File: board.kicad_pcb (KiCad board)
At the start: 4 copper layers, 50 x 50 mm, 47 parts, among them J1 TEMPS, J2 OLED, J3 HV1, J4 HV2, J5 PWR_IN, J6 PROG, K1 RELAY1, K3 RELAY2, Q3 AO3400A, Q4 AO3400A, U1 ESP32-WROOM-32, U2 AMS1117, U3 USB3_1C16PFSMT, U4 CH340E, U5 SW_RST, U6 SW_BOOT

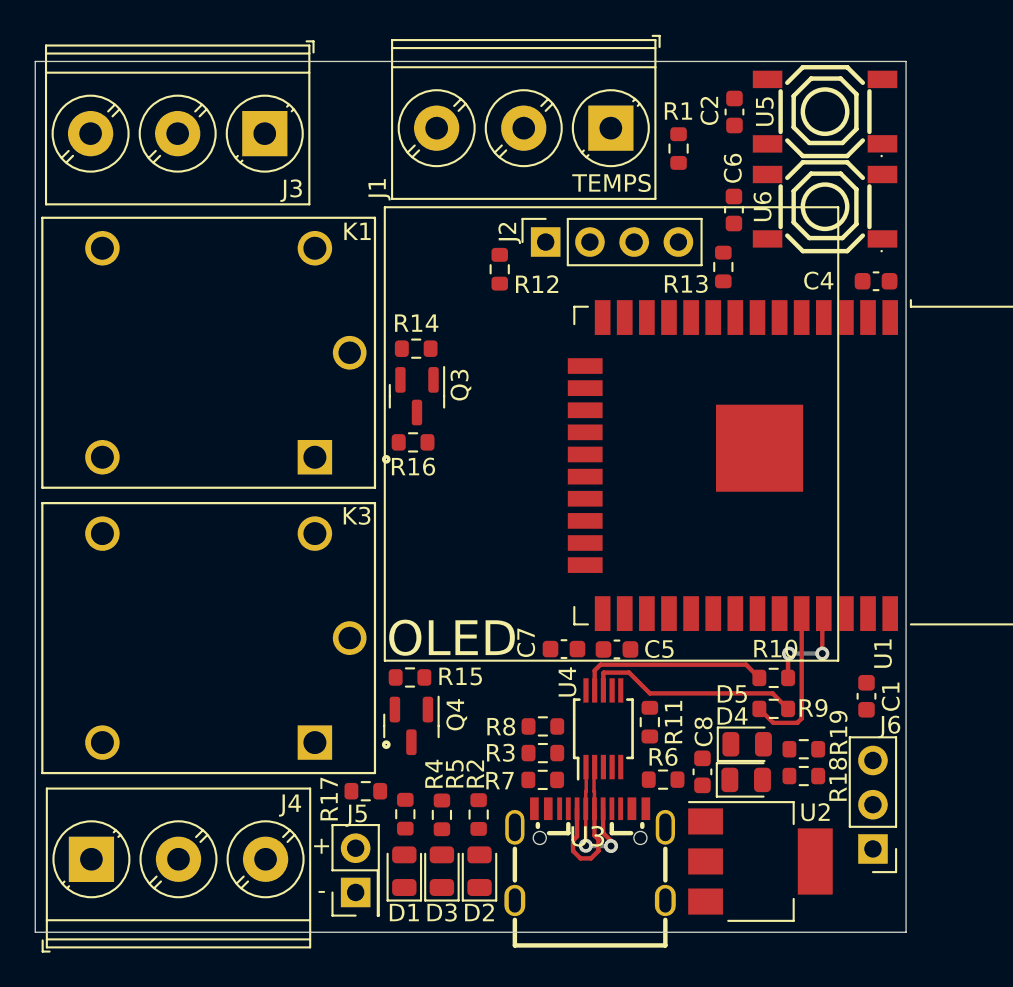
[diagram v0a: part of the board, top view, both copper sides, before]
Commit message: feat: initial routing
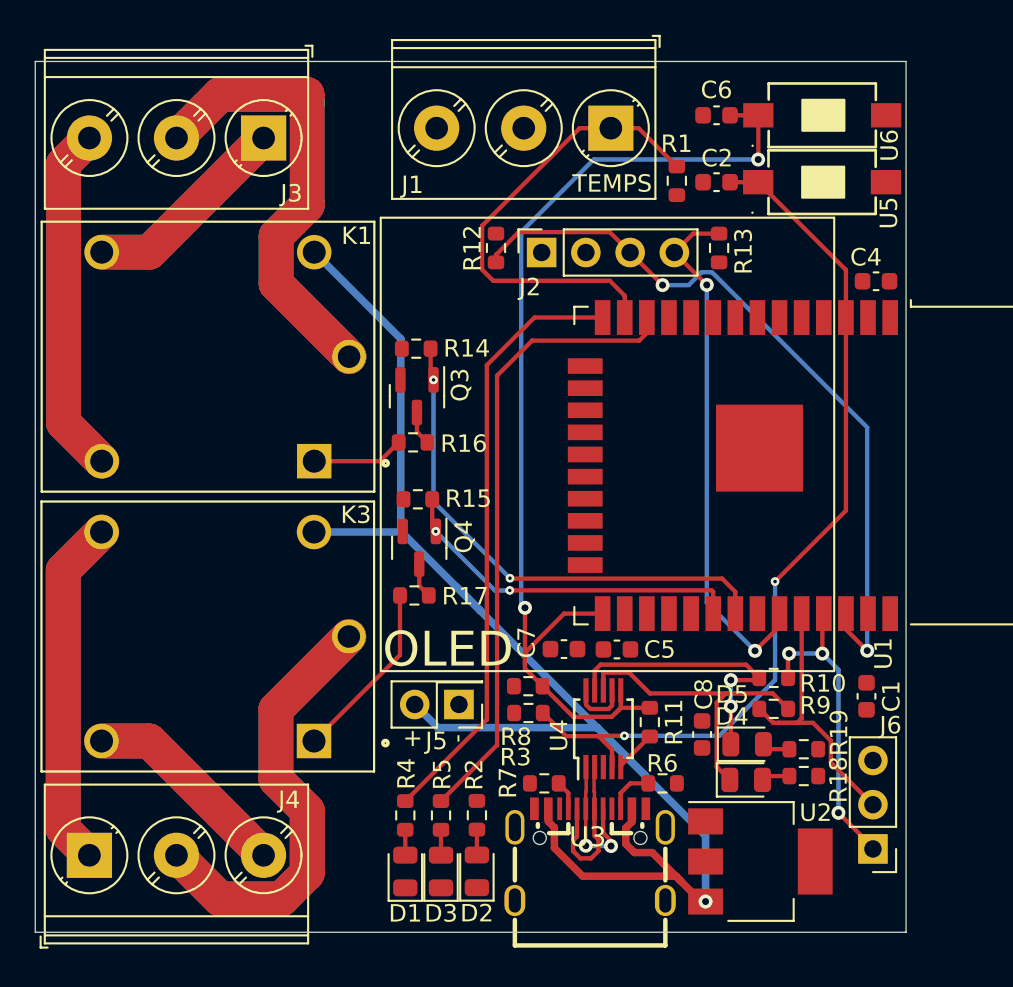
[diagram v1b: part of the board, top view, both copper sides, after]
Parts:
- J3: value HV1 -> HV2
- J4: value HV2 -> HV1
- K1: value RELAY1 -> RELAY2
- K3: value RELAY2 -> RELAY1
- U2: value AMS1117 -> AMS1117-3.3
- U5, U6: footprint board:SW-SMD_4P-L5.1-W5.1-P3.70-LS6.5-TL-2 -> board:SW-SMD_L6.0-W3.5-LS8.0
- moved J5 12.3 mm to (78.8, 140.2), turned to 180 degrees
- moved R17 11.6 mm to (76.3, 133.9)
- moved Q4 10.2 mm to (76.5, 131.2)
- moved R15 10.2 mm to (76.5, 128.4)
- moved C6 5.53 mm to (93.6, 106.4), turned to 0 degrees
- moved U6 5.25 mm to (99.7, 106.4), turned to 0 degrees
- moved C2 4.16 mm to (93.6, 110.2), turned to 0 degrees
- moved U5 4.05 mm to (99.7, 110.2), turned to 0 degrees
- moved R8 2.46 mm to (82.8, 139.2)
- moved R3 2.45 mm to (82.8, 140.7)
- moved C8 2.15 mm to (92.8, 141.9)
- moved R1 1.85 mm to (91.3, 110.1)
- moved R12 1.24 mm to (81.0, 114.0)
- moved R13 1.12 mm to (93.8, 114.0)
- moved J2 0.64 mm to (83.6, 114.3)
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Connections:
- Q3 pad 1: CH1 -> CH2
- Q4 pad 1: CH2 -> CH1
- R14 pad 2: CH1 -> CH2
- R15 pad 2: CH2 -> CH1
- U5 pad 2: EN_ESP -> GND
- U6 pad 2: GPIO0 -> GND
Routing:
- net Net-(J3-Pad2): track 0.00 -> 103.2 mm
- net Net-(J4-Pad2): track 0.00 -> 100.9 mm
- net VBUS: track 0.00 -> 87.0 mm, vias 0 -> 1
- net Net-(J4-Pad1): track 0.00 -> 80.4 mm
- net Net-(J3-Pad3): track 0.00 -> 80.3 mm
- net GPIO0: track 0.00 -> 60.6 mm, vias 0 -> 2
- net EN_ESP: track 0.00 -> 51.3 mm, vias 0 -> 2
- net Net-(J4-Pad3): track 0.00 -> 48.1 mm
- net Net-(J3-Pad1): track 0.00 -> 48.0 mm
- net SCL: track 0.00 -> 43.0 mm, vias 0 -> 2
- net SLED2: track 0.00 -> 36.3 mm
- net SLED1: track 0.00 -> 34.7 mm
- net SDA: track 0.00 -> 30.5 mm, vias 0 -> 2
- net CH2: track 0.00 -> 29.6 mm, vias 0 -> 2
- net GPIO14: track 0.00 -> 27.0 mm
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
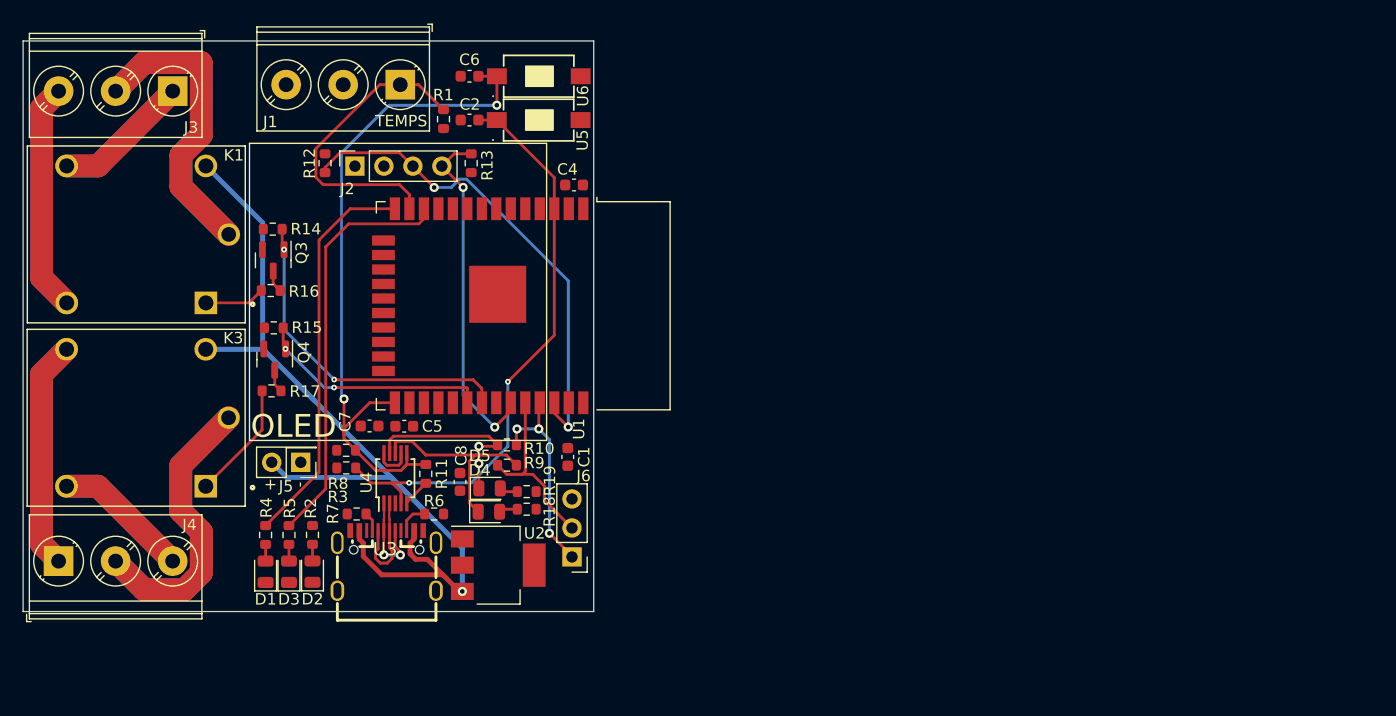
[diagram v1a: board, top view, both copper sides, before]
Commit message: feat: routed with planes and no warnings or errors
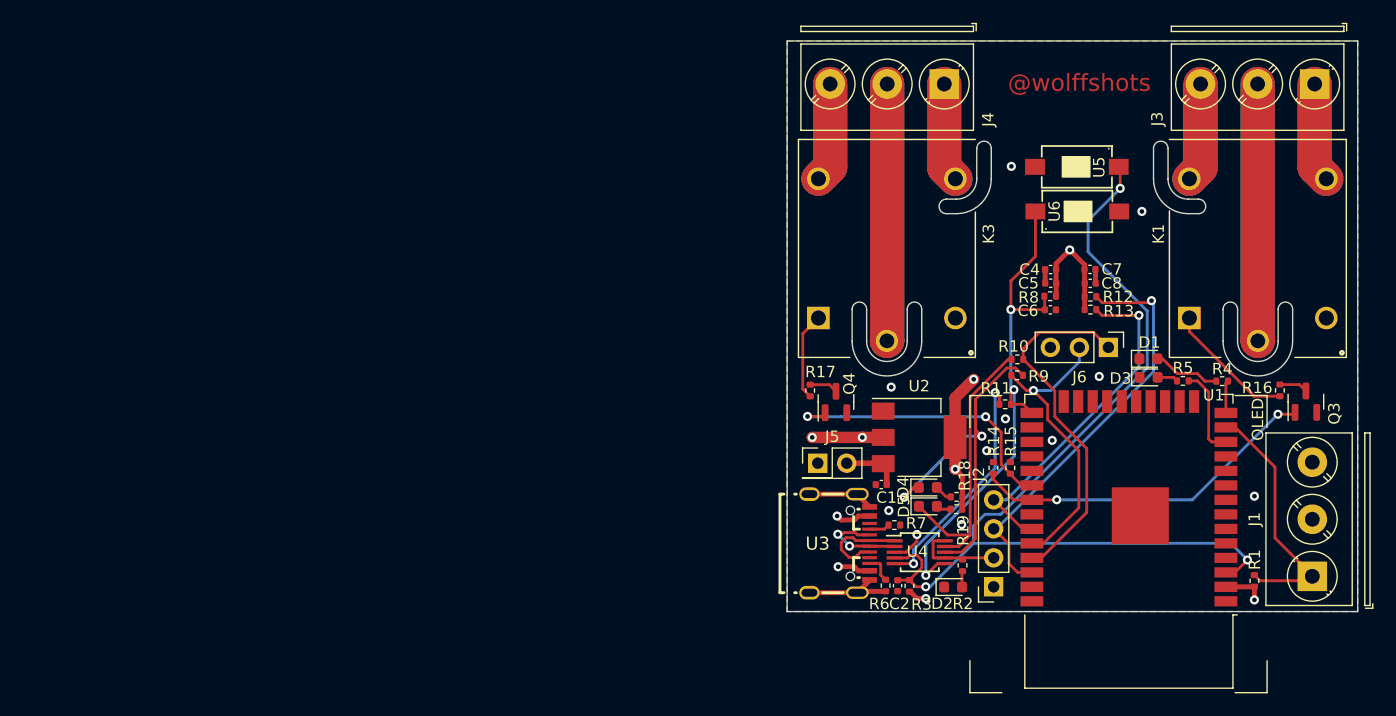
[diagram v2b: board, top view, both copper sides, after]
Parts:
- C1, C2, C4, C5, C6, C7, C8: footprint Capacitor_SMD:C_0603_1608Metric -> Capacitor_SMD:C_0402_1005Metric
- D1, D2, D3, D4, D5: footprint LED_SMD:LED_0805_2012Metric -> LED_SMD:LED_0603_1608Metric
- R1, R10, R11, R12, R13, R14, R15, R16, R17, R18, R19, R2, R3, R4, R5, R6, R7, R8, R9: footprint Resistor_SMD:R_0603_1608Metric -> Resistor_SMD:R_0402_1005Metric
- U3: value USB3_1C16PFSMT -> USBC
- moved J3 100.1 mm to (167.7, 107.1)
- moved K1 98.5 mm to (163.0, 120.2), turned to 0 degrees
- moved Q3 91.3 mm to (166.9, 134.9), turned to 90 degrees
- moved J1 90.8 mm to (167.5, 150.2), turned to 90 degrees
- moved R16 88.9 mm to (164.6, 133.9), turned to -90 degrees
- moved J4 88.2 mm to (135.2, 107.1), turned to 180 degrees
- moved R4 84.9 mm to (159.6, 133.1), turned to 180 degrees
- moved R1 81.8 mm to (162.4, 150.6)
- moved D1 79.6 mm to (153.1, 131.1), turned to 0 degrees
- moved R5 79.5 mm to (156.1, 133.1), turned to 180 degrees
- moved D3 77.2 mm to (153.1, 132.8), turned to 0 degrees
- moved R12 68.1 mm to (148.0, 125.7), turned to 0 degrees
- moved K3 68.0 mm to (130.4, 120.2), turned to 0 degrees
- moved J2 67.0 mm to (139.6, 151.1), turned to 180 degrees
- moved R14 66.5 mm to (139.5, 140.7), turned to -90 degrees
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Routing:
- net Net-(J4-Pad1): track 80.4 -> 34.9 mm
- net Net-(J3-Pad3): track 80.3 -> 34.9 mm
- net +3V3: track 3.37 -> 42.2 mm, vias 0 -> 7
- net EN_ESP: track 51.3 -> 83.7 mm, vias 2 -> 3
- net SLED1: track 34.7 -> 2.86 mm
- net SLED2: track 36.3 -> 7.88 mm
- net GND: track 0.00 -> 19.4 mm, vias 0 -> 11
- net NCTS: track 2.45 -> 20.8 mm, vias 0 -> 2
- net TX_CH: track 19.0 -> 35.1 mm, vias 0 -> 2
- net GPIO0: track 60.6 -> 45.9 mm, vias 2 -> 3
- net TX_ESP: track 18.1 -> 31.7 mm, vias 3 -> 0
- net Net-(J4-Pad3): track 48.1 -> 34.9 mm
- net Net-(J3-Pad2): track 103.2 -> 90.1 mm
- net Net-(J3-Pad1): track 48.0 -> 34.9 mm
- net Net-(J4-Pad2): track 100.9 -> 90.1 mm
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- added copper zone on In2.Cu, net +3V3
- added copper zone on B.Cu, net GND
- added copper zone on F.Cu, net GND
- added copper zone on In1.Cu, net GND
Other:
- board text added: "@wolffshots"
